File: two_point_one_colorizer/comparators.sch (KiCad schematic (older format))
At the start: 13 parts, among them U8 LM393

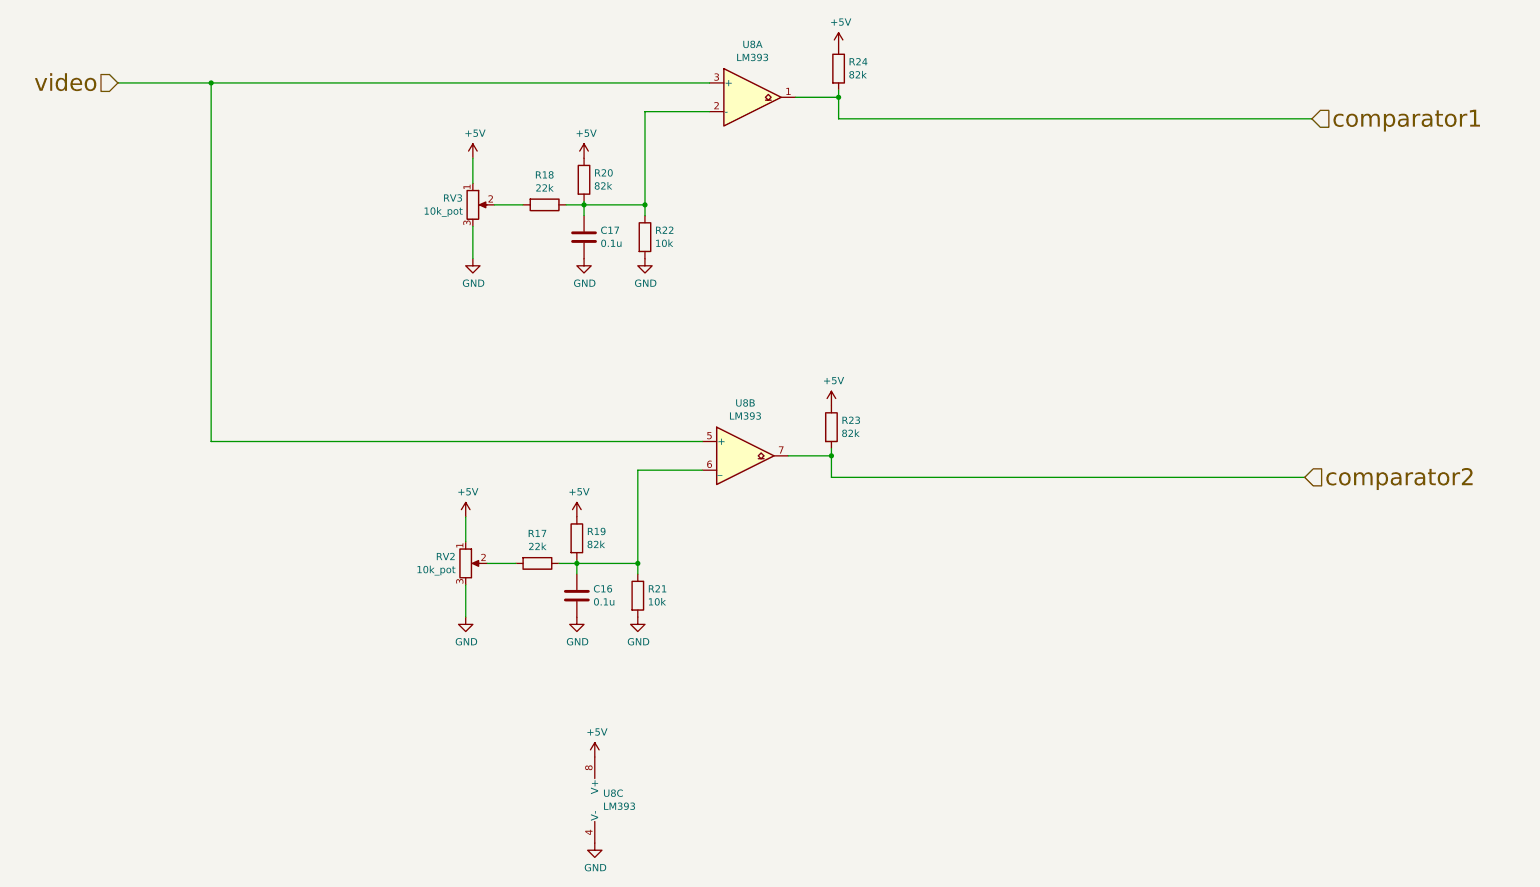
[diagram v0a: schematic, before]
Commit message: updates
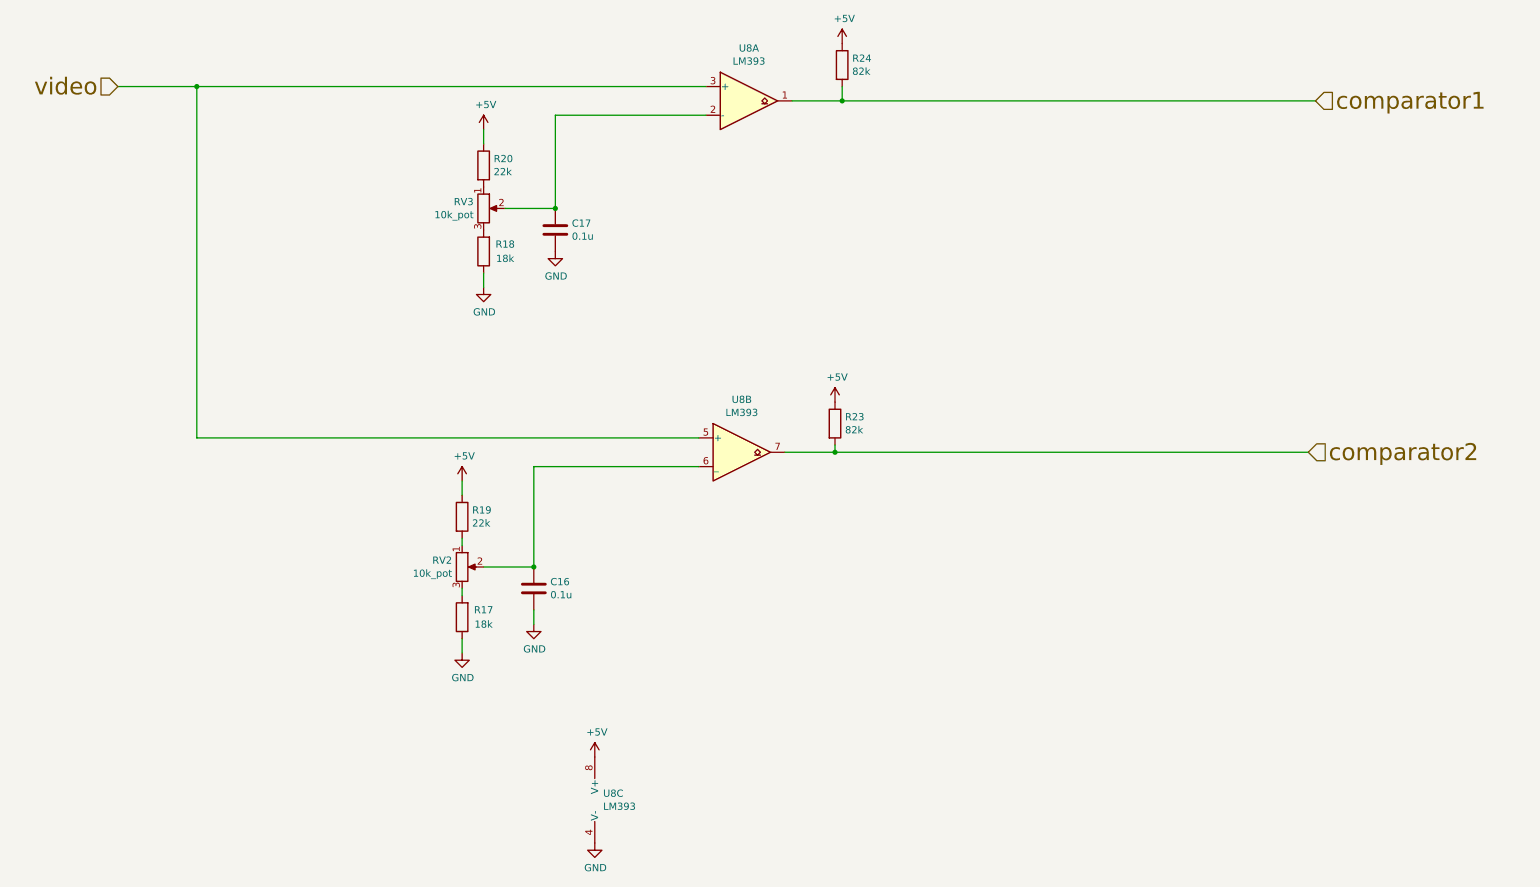
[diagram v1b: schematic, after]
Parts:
- removed R21, R22: 10k, lib_fp:R_Axial_DIN0207_L6.3mm_D2.5mm_P7.62mm_Horizontal, symbol Device:R
- R17, R18: value 22k -> 18k
- R19, R20: value 82k -> 22k
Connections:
- net +5V: no longer RV2.1, RV3.1
- net GND: now also R17.1, R18.1; no longer RV2.3, RV3.3
- net at RV3.2: now also C17.1, U8.2 (-); no longer R18.2
- net at RV2.2: now also C16.1, U8.6 (_); no longer R17.2
- new net: R20.2, RV3.1
- new net: R18.2, RV3.3
- new net: R19.2, RV2.1
- new net: R17.2, RV2.3
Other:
- moved on the sheet: C16, C17, R17, R18, R19, R20, R23, R24, RV2, RV3, U8A, U8B
